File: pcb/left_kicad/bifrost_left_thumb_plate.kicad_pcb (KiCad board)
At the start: 2 copper layers, 61.2 x 39.5 mm, 3 parts

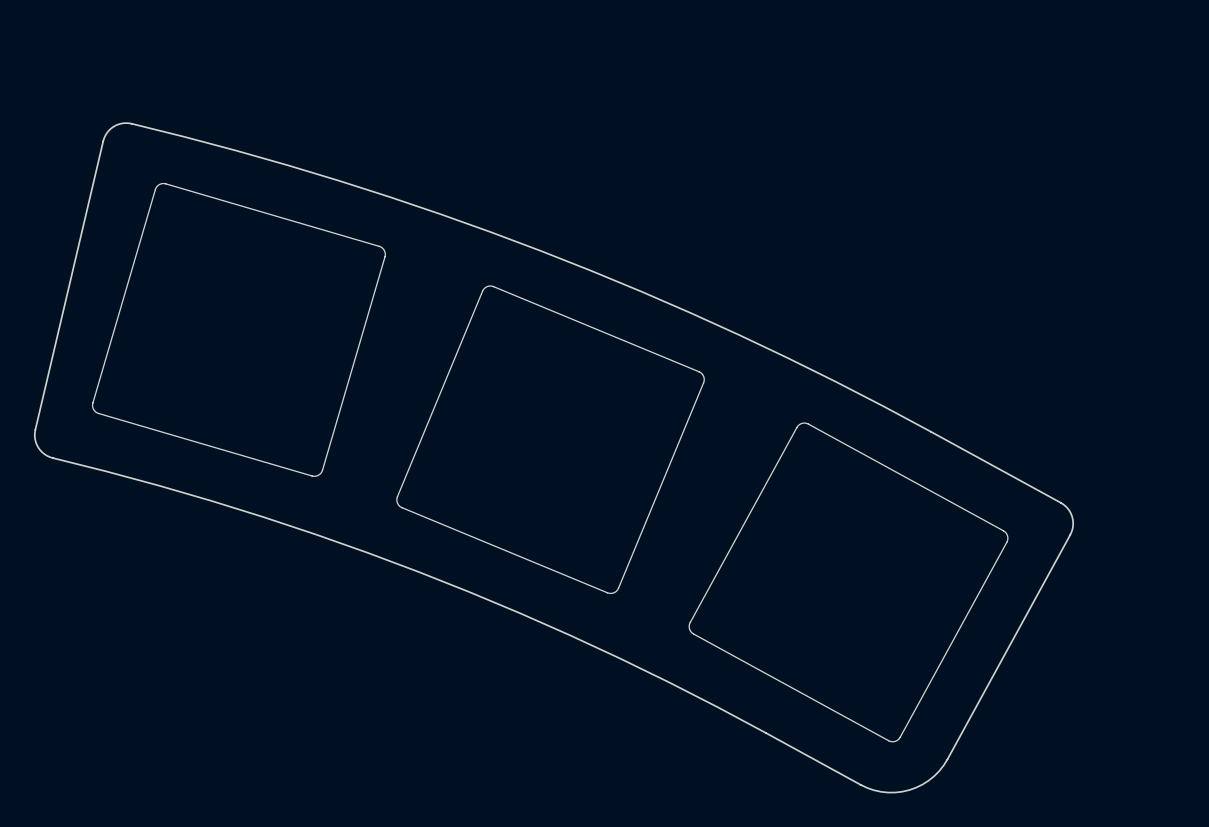
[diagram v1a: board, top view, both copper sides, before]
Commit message: Update PCB and case designs
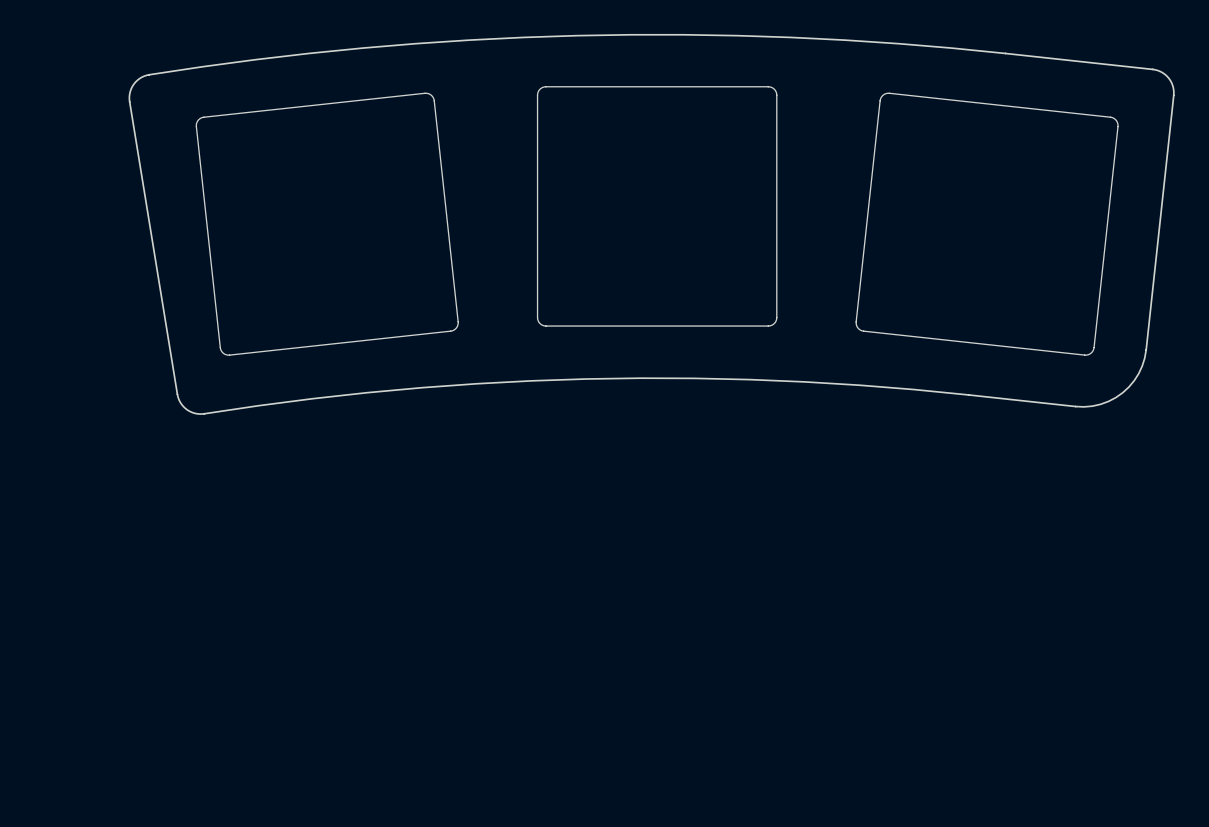
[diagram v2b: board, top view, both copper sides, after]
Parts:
- PH41: value R0C40 -> 1U
- PH42: value R0C41 -> 1U
- PH43: value R0C42 -> 1U
- moved PH43 22.6 mm to (118.7, 60.6), turned to -6.179 degrees
- moved PH42 15.1 mm to (99.2, 59.5), turned to 0 degrees
- moved PH41 8.12 mm to (79.8, 60.6), turned to 6.179 degrees
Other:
- board size 61.2 x 39.5 mm -> 61.6 x 22.4 mm
